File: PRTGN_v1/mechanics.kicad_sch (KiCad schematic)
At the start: 15 parts, among them SW5 SW_Push, SW6 SW_Push, SW7 SW_Push, SW8 SW_Push

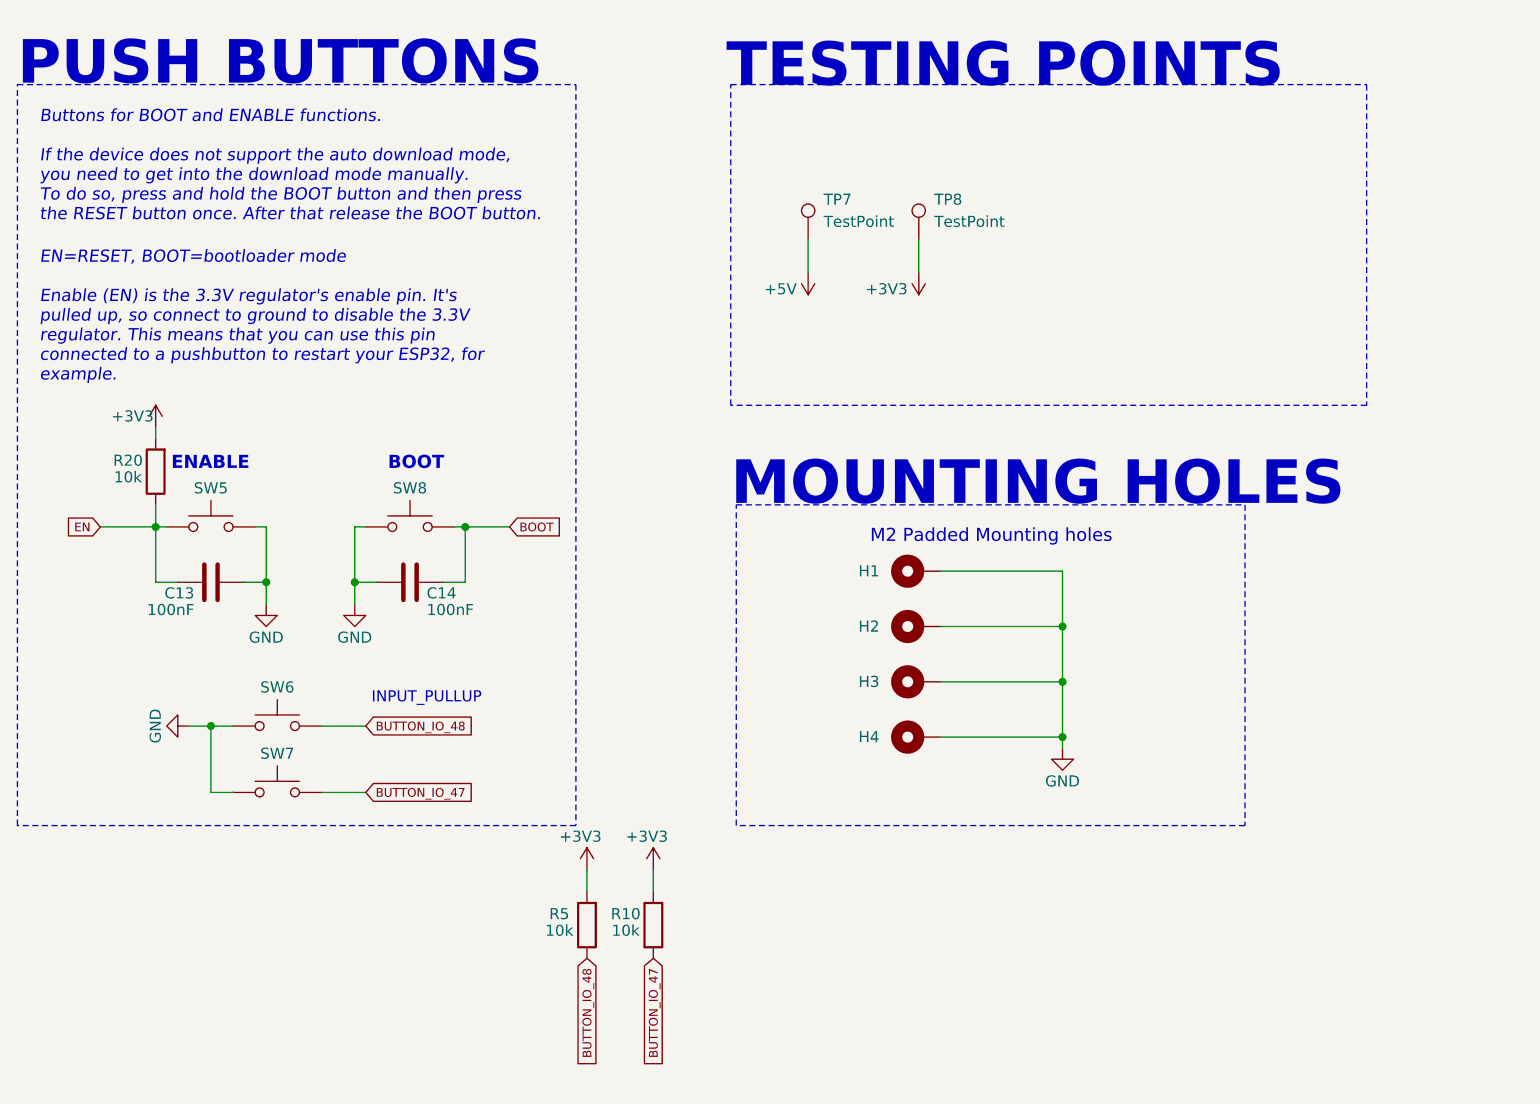
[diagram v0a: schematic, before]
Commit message: upd
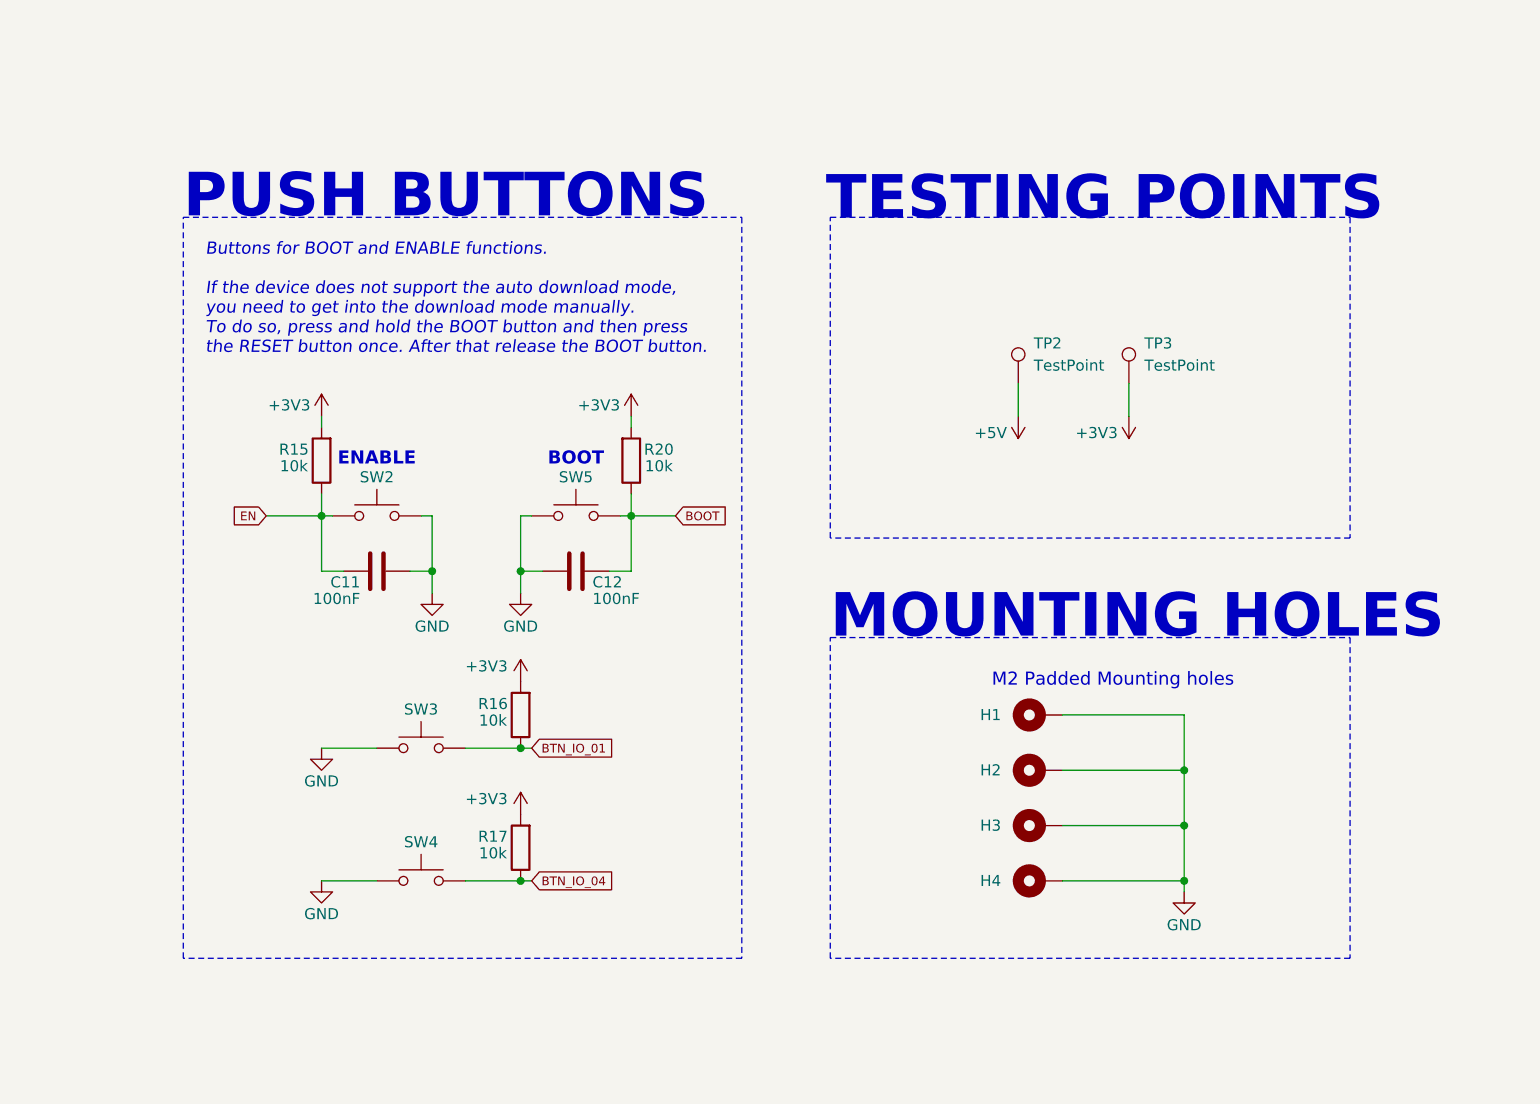
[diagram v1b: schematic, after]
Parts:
- added R20: 10k, Resistor_SMD:R_0805_2012Metric_Pad1.20x1.40mm_HandSolder, symbol Device:R
- renumbered C13 to C11, C14 to C12, R20 to R15, R5 to R16, R10 to R17, SW5 to SW2, SW6 to SW3, SW7 to SW4, SW8 to SW5, TP7 to TP2, TP8 to TP3
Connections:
- net +3V3: now also R20.2
- net BOOT: now also R20.1
- net BUTTON_IO_47 renamed BTN_IO_04
- net BUTTON_IO_48 renamed BTN_IO_01
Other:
- note removed: "EN=RESET, BOOT=bootloader mode Enable (EN) is the 3.3V regulator's enable pin. It's pulled up, so connect to ground to disable the 3.3V regulator. This means that you can use this pin connected to a pushbutton to restart your ESP32, for example."
- note removed: "INPUT_PULLUP"
- moved on the sheet: C11, C12, H1, H2, H3, H4, R15, R16, R17, SW2, SW3, SW4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
